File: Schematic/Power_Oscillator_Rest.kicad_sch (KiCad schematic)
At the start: 33 parts, among them J1 Barrel_Jack_Switch_Pin3Ring, SW1 SW_DPDT_x2, SW2 SW_Push, SW3 SW_Push, U1 L7805, U2 ATF16V8B, U4 74LS373, U6 M48Z35, U8 74LS374, Y1 Crystal (11.0592 MHz)

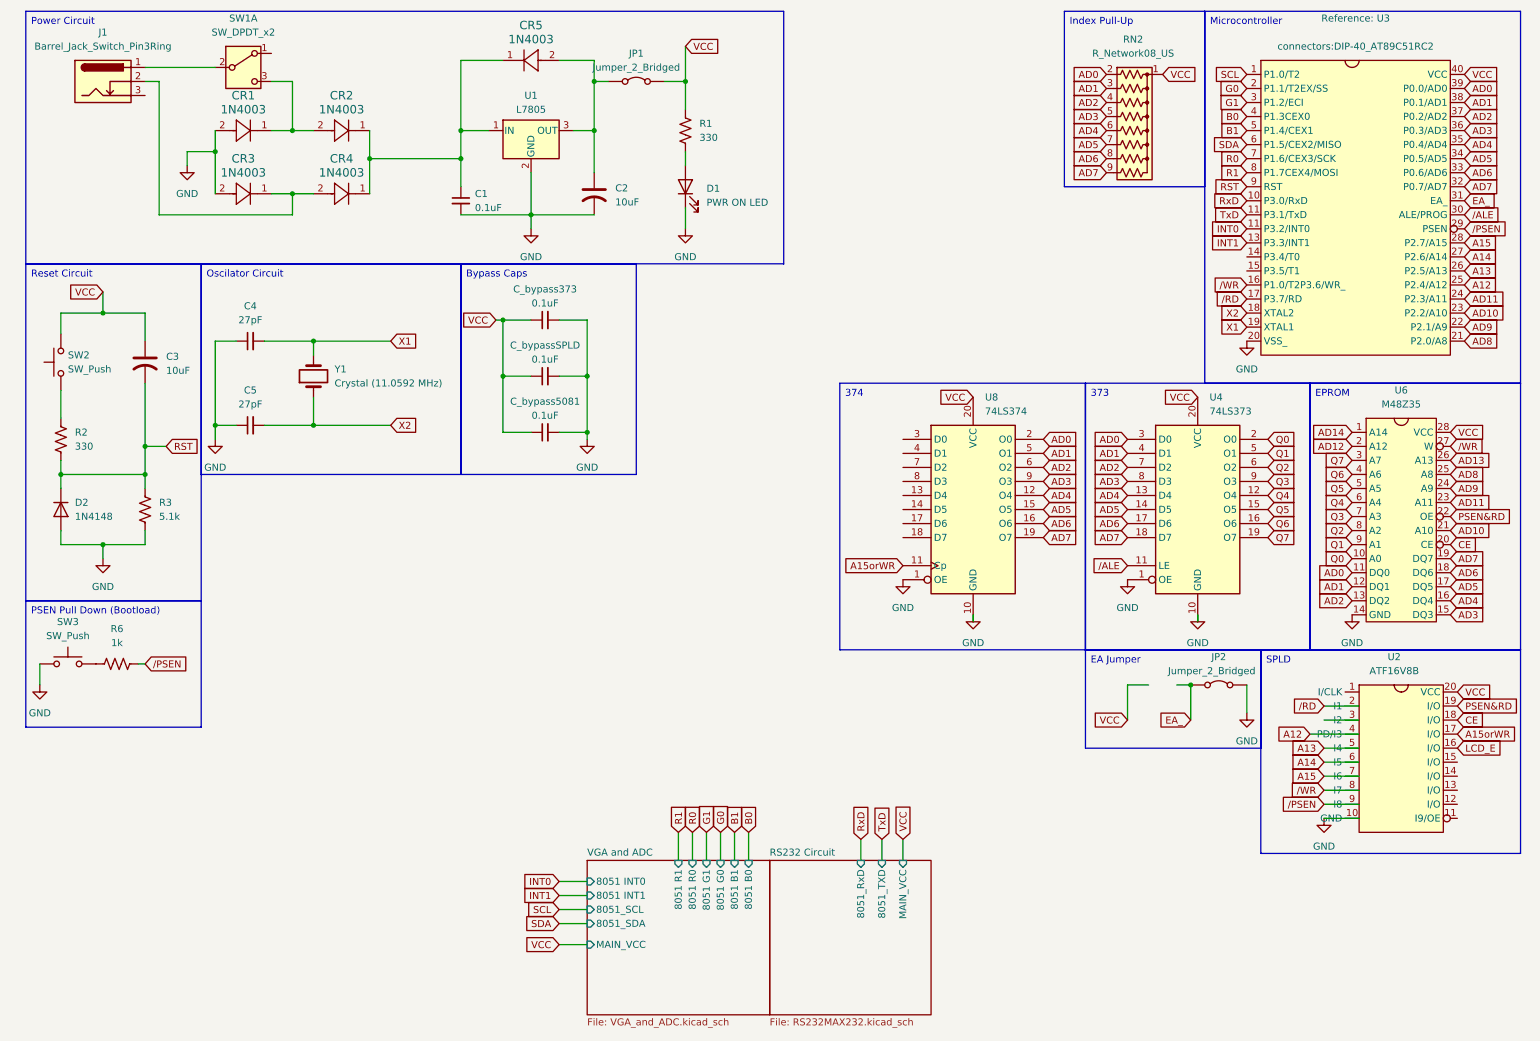
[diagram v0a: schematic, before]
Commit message: updated make and circuit
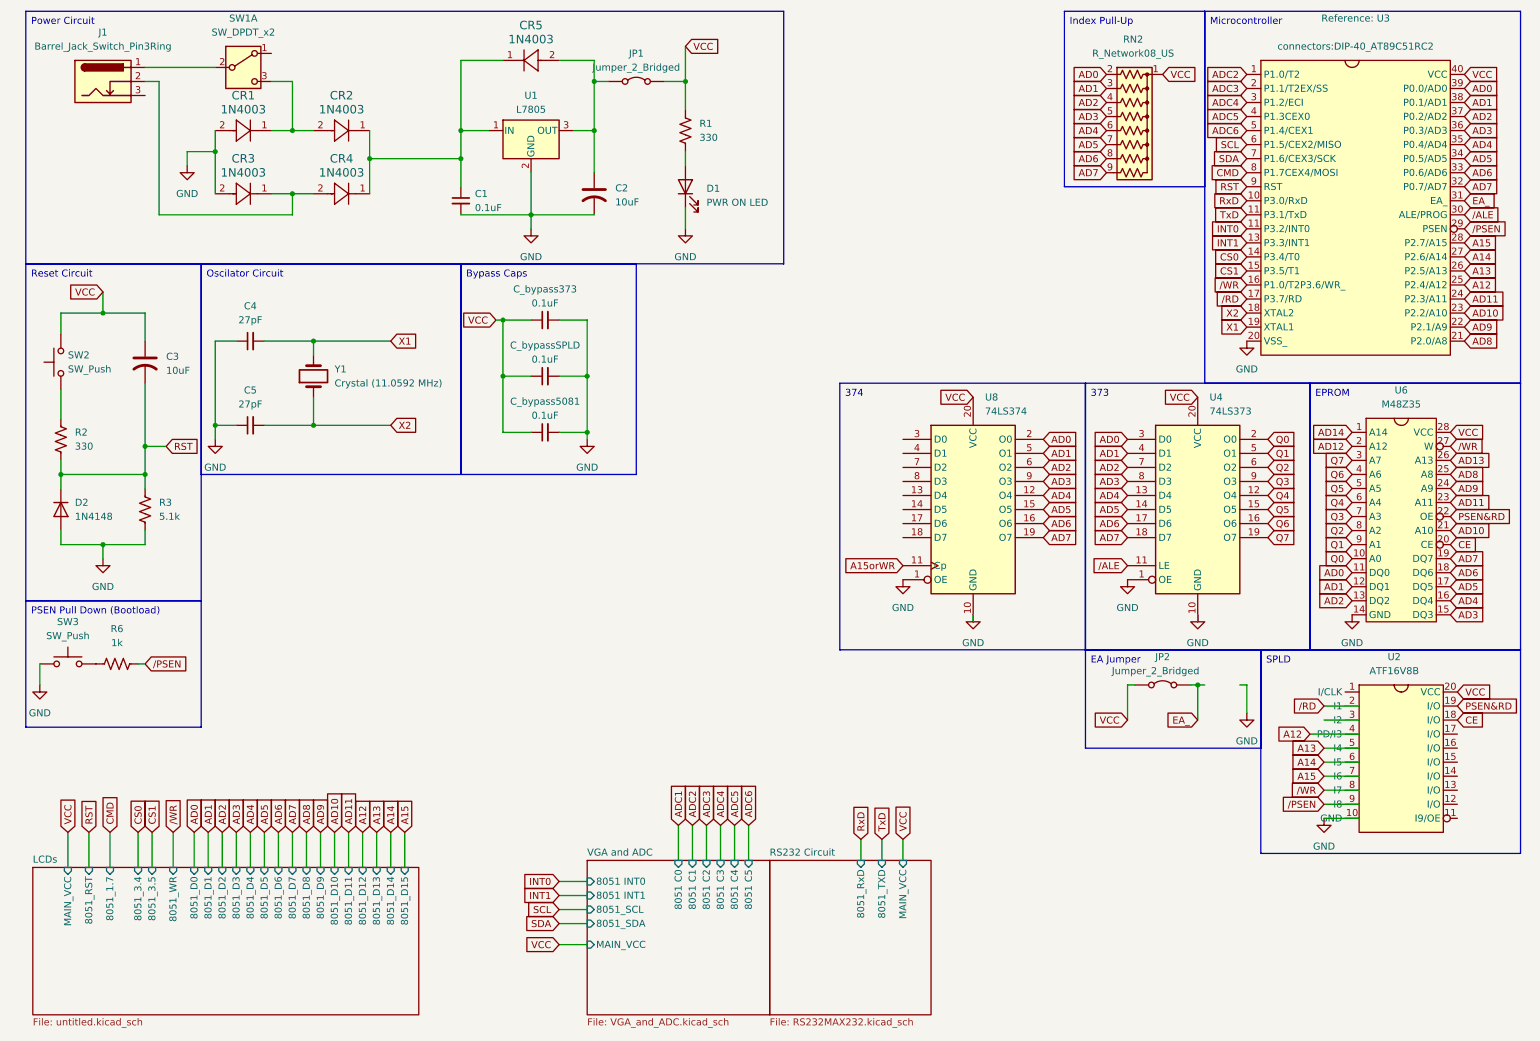
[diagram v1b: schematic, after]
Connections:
- net R0 is gone; now on net SDA: U3.7 (P1.6/CEX3/SCK)
- net A15orWR: no longer U2.17 (I/O)
- net EA_: now also JP2.2 (B); no longer JP2.1 (A)
- net GND: no longer JP2.2 (B)
- net SCL: now also U3.6 (P1.5/CEX2/MISO); no longer U3.1 (P1.0/T2)
- net SDA: no longer U3.6 (P1.5/CEX2/MISO)
- net VCC: now also JP2.1 (A)
- net CS0: now reaches U3.14 (P3.4/T0)
- net CS1: now reaches U3.15 (P3.5/T1)
- net B0 renamed ADC5
- net B1 renamed ADC6
- net G0 renamed ADC3
- net G1 renamed ADC4
- net LCD_E: no longer names the net of U2.16 (I/O)
- net R1 renamed CMD
- new net ADC2: U3.1 (P1.0/T2)
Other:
- added sheet LCDs (untitled.kicad_sch)
- sheet VGA and ADC ports: added 8051 C0, 8051 C1, 8051 C2, 8051 C3, 8051 C4, 8051 C5; removed 8051 B0, 8051 B1, 8051 G0, 8051 G1, 8051 R0, 8051 R1
- moved on the sheet: JP2
